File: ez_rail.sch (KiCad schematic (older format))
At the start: 16 parts, among them J1 Conn_01x02_Male, J2 Conn_01x02_Male, J3 Conn_01x03_Male, U1 LM2575T, U2 LM2575T

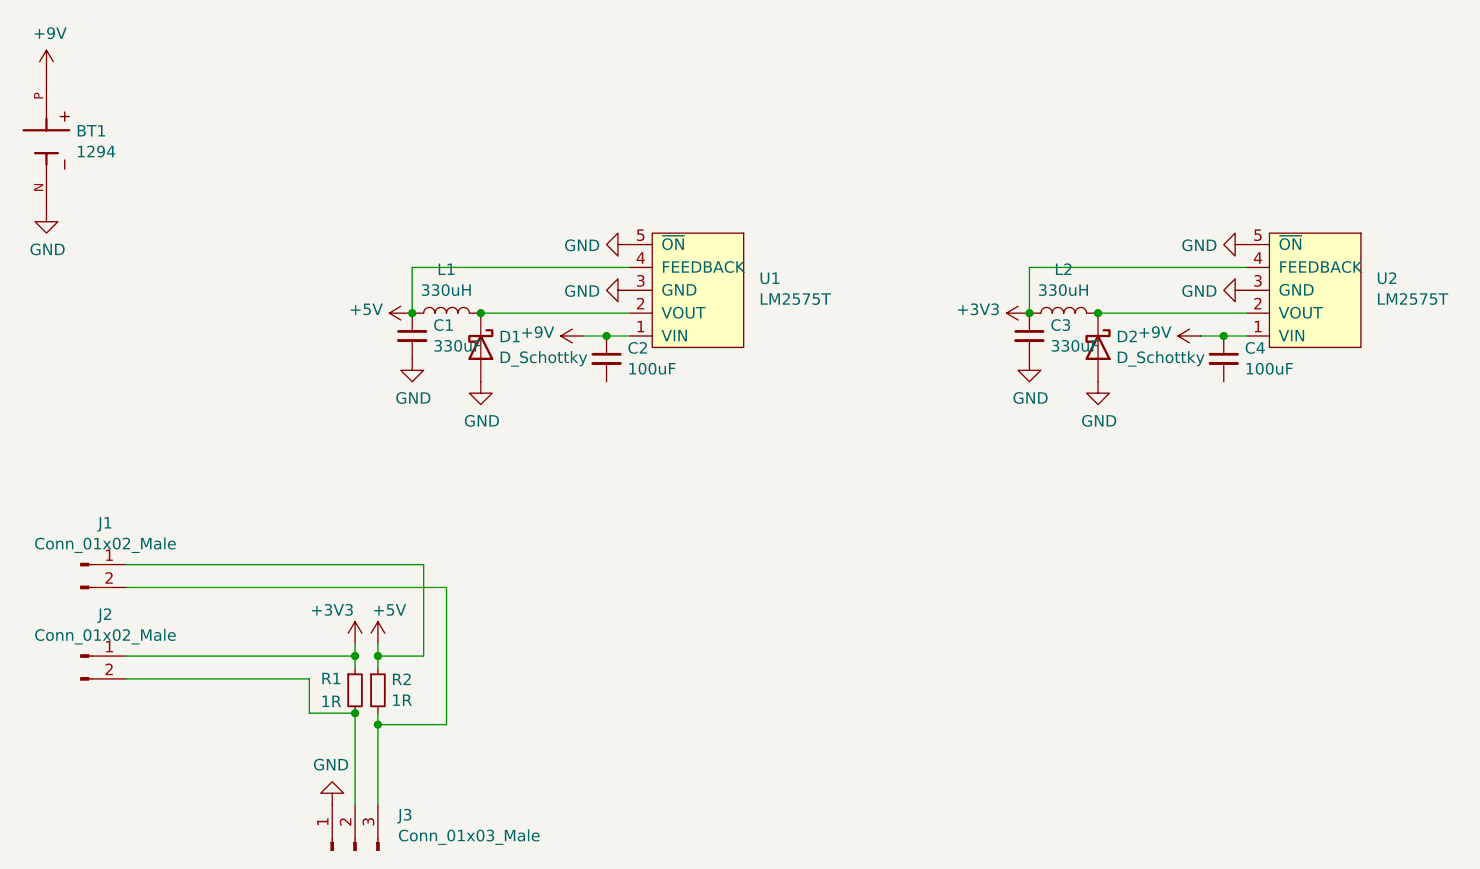
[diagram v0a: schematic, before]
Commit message: Finishing layout, adding gitignore, removing cache file
Adding media & readme
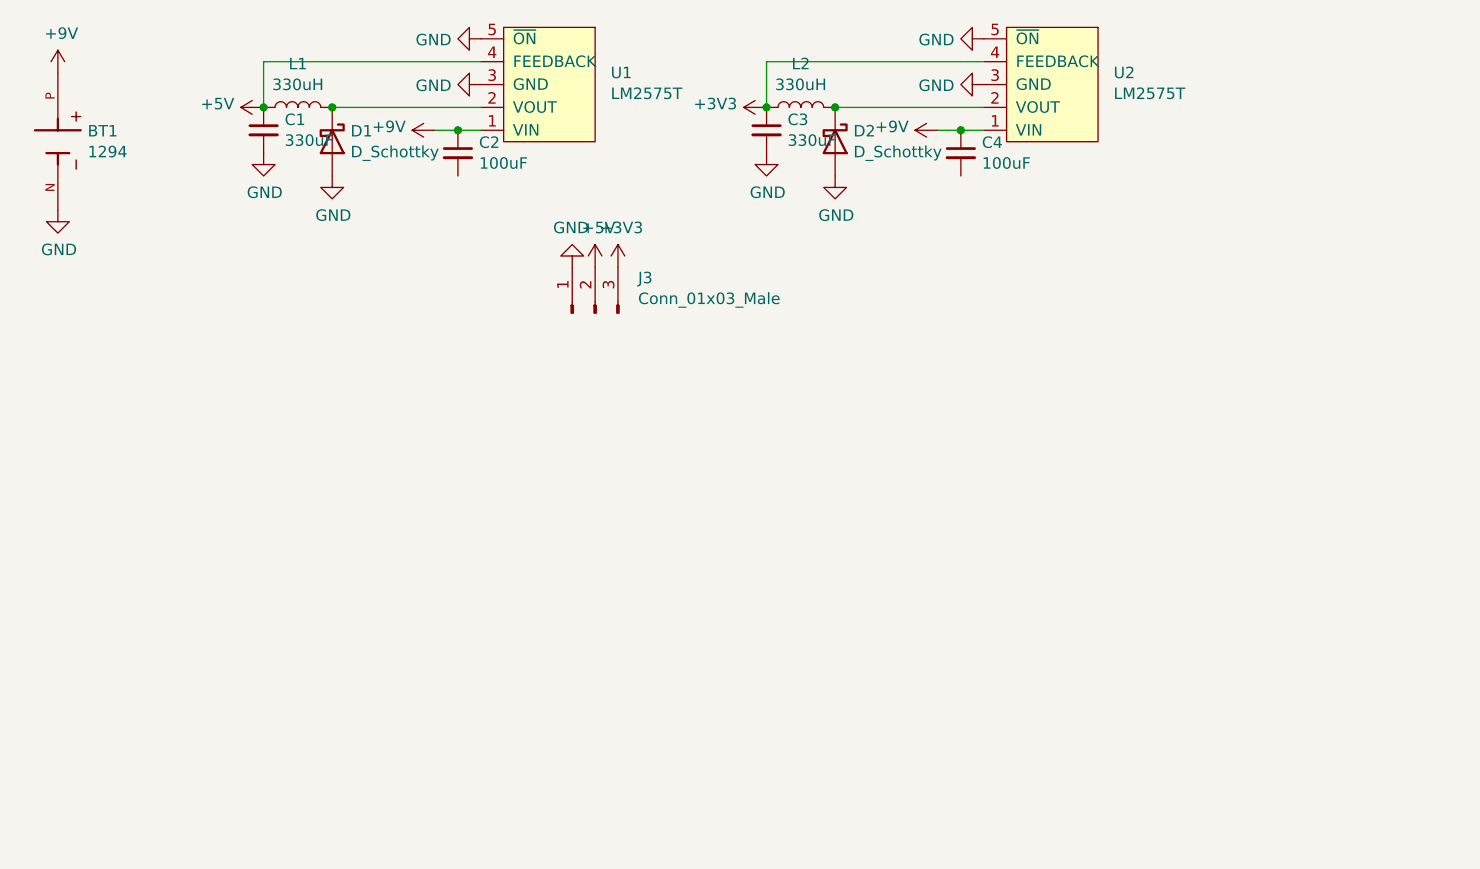
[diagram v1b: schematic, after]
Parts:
- removed J1, J2: Conn_01x02_Male, Connector_PinHeader_2.54mm:PinHeader_1x02_P2.54mm_Vertical, symbol Connector:Conn_01x02_Male
- removed R1, R2: 1R, Resistor_THT:R_Axial_DIN0614_L14.3mm_D5.7mm_P15.24mm_Horizontal, symbol Device:R_Small
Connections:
- net +3V3: now also J3.3 (Pin_3)
- net +5V: now also J3.2 (Pin_2)
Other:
- moved on the sheet: BT1, C1, C2, C3, C4, D1, D2, J3, L1, L2, U1, U2
